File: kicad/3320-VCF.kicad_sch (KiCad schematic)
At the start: 65 parts, among them J1 EuroPower_JST_3P, J2 EURO_PWR_16P, U1 TL072, U2 TL074, U3 AS3320

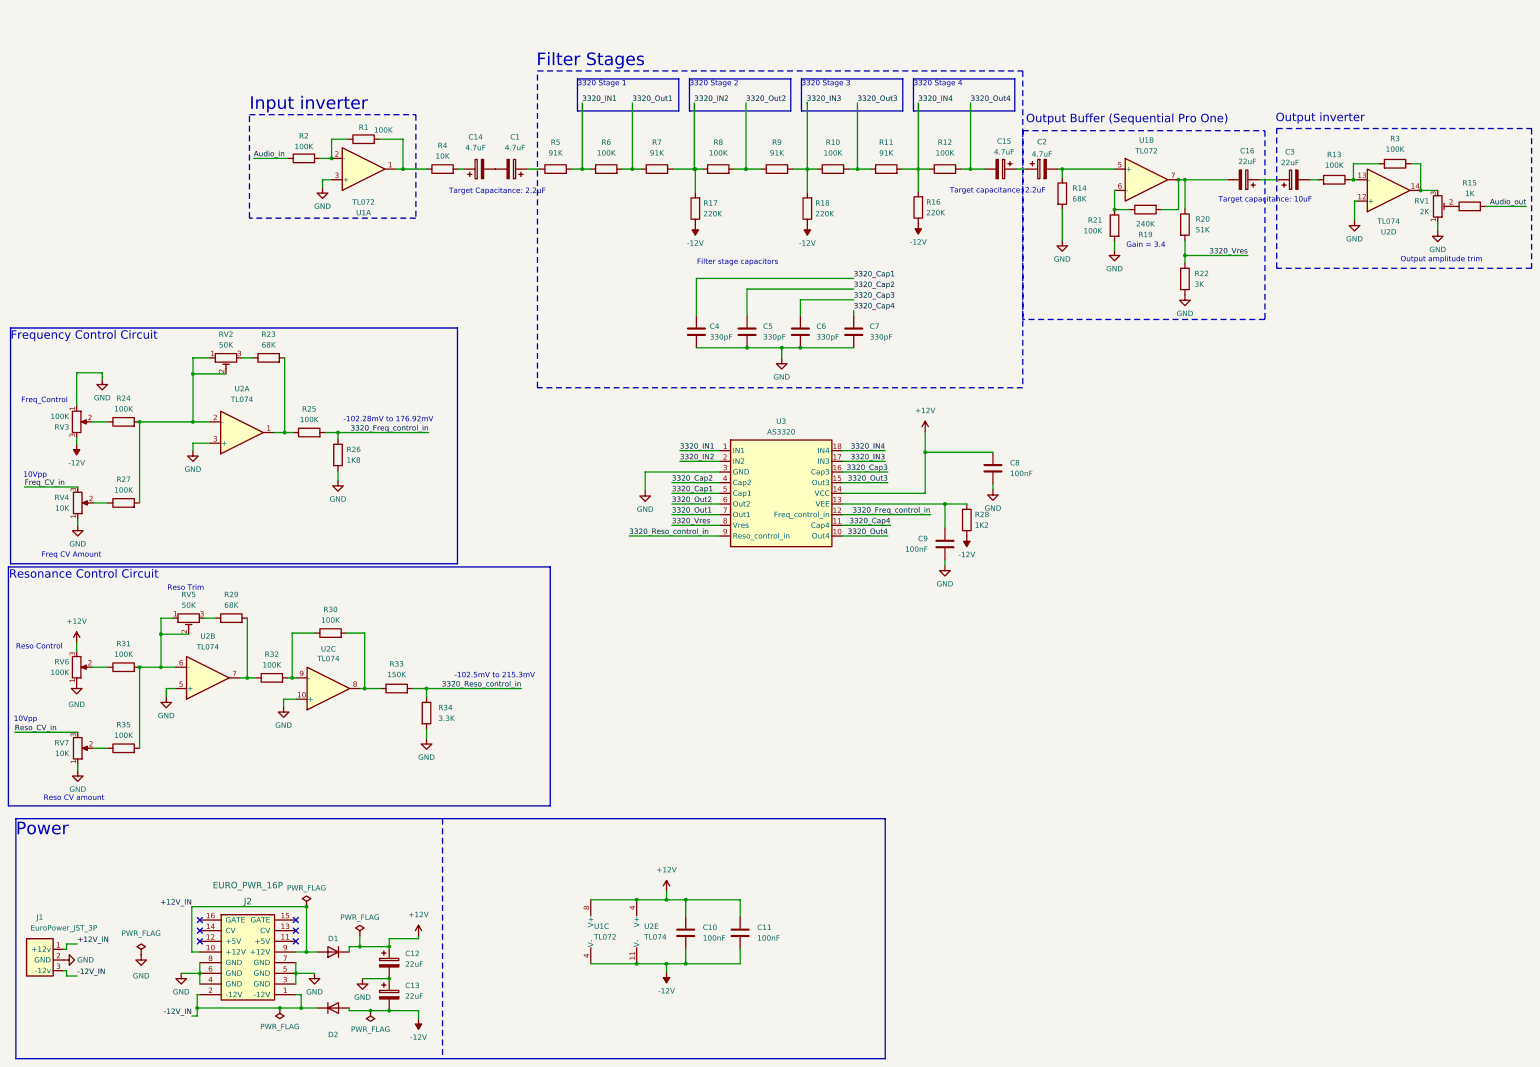
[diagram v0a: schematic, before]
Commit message: Added Schematic Revision 0.1.1
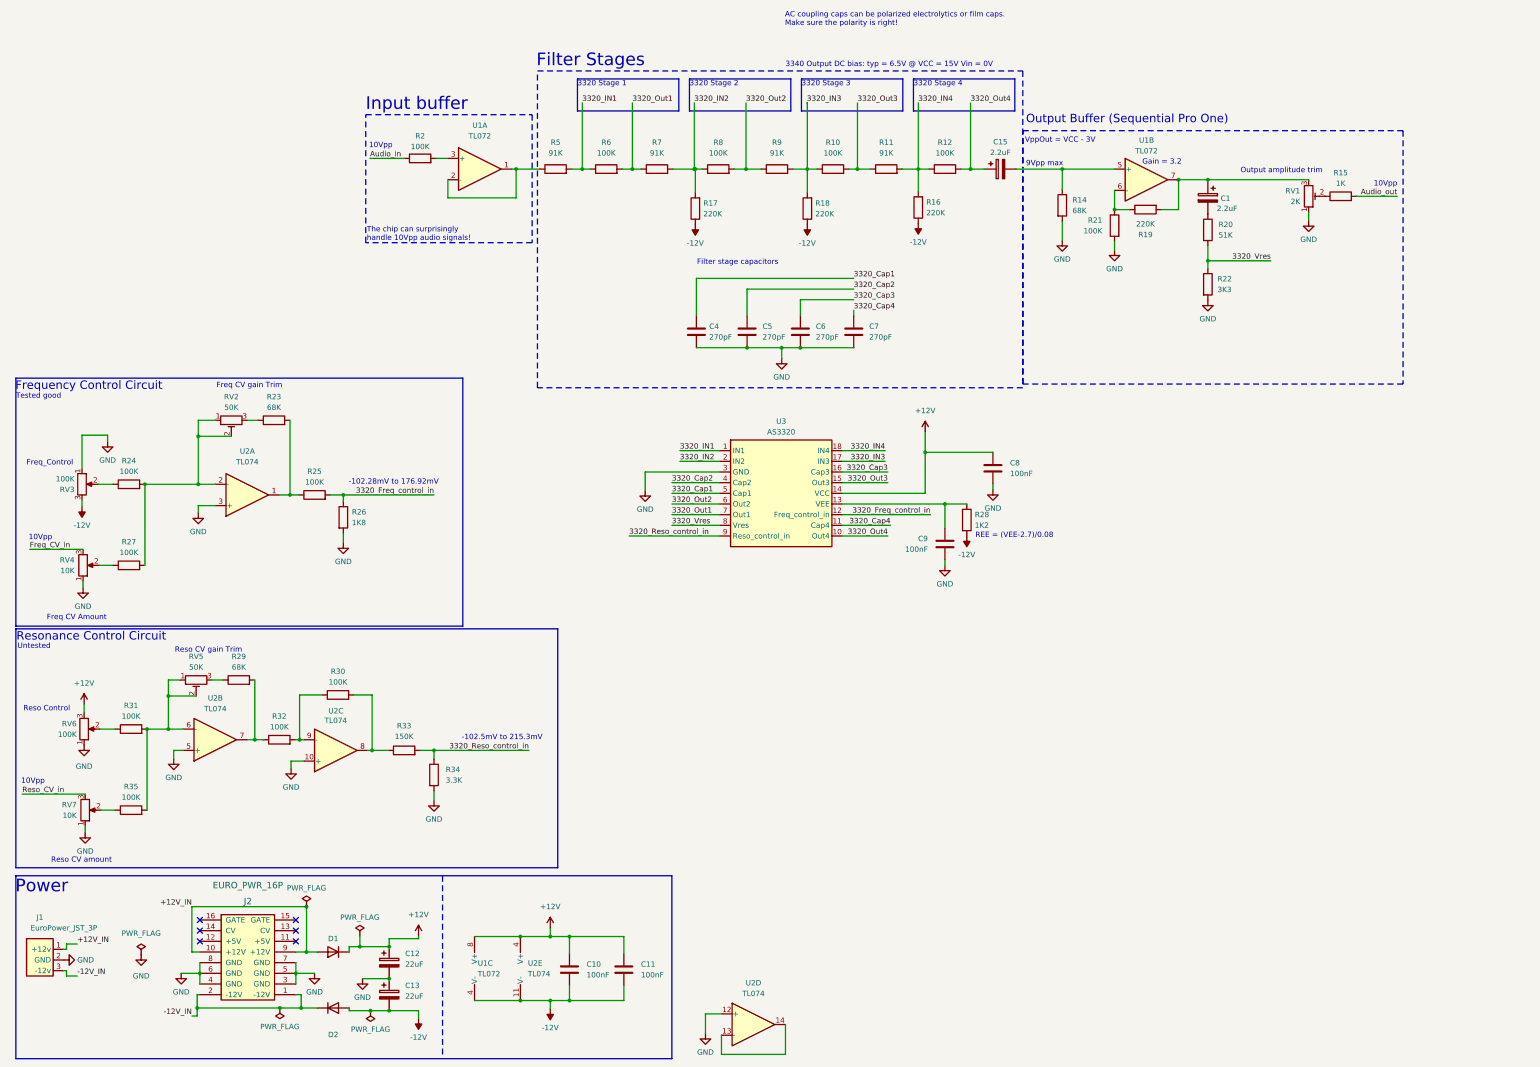
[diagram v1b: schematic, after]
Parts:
- removed C14, C2: 4.7uF, symbol Device:C_Polarized
- removed C16, C3: 22uF, symbol Device:C_Polarized
- removed R1, R13, R3: 100K, symbol Device:R
- removed R4: 10K, symbol Device:R
- C1, C15: value 4.7uF -> 2.2uF
- C4, C5, C6, C7: value 330pF -> 270pF
- R19: value 240K -> 220K
- R22: value 3K -> 3K3
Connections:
- net 3320_Out4: now also C15.1; no longer C15.2
- net GND: no longer U1.3 (+)
- net at R14.1, U1.5 (+): now also C15.2
- net at C1.2: now also R20.1
- net at U1.1: now also R5.1, U1.2 (-)
- net at U2.13 (-): now also U2.14
- net at C1.1: now also R19.2, RV1.3, U1.7; no longer R5.1
- net at R2.2: now also U1.3 (+); no longer U1.2 (-)
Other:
- note added: "3340 Output DC bias: typ = 6.5V @ VCC = 15V Vin = 0V"
- note added: "9Vpp max"
- note added: "AC coupling caps can be polarized electrolytics or film caps. Make sure the polarity is right!"
- note added: "Freq CV gain Trim"
- note added: "Gain = 3.2"
- note added: "Input buffer"
- note added: "REE = (VEE-2.7)/0.08"
- note added: "Reso CV gain Trim"
- note added: "Tested good"
- note added: "The chip can surprisingly handle 10Vpp audio signals!"
- note added: "Untested"
- note added: "VppOut = VCC - 3V"
- note removed: "Gain = 3.4"
- note removed: "Input inverter"
- note removed: "Output inverter"
- note removed: "Reso Trim"
- note removed: "Target Capacitance: 2.2uF"
- note removed: "Target capacitance: 10uF"
- note removed: "Target capacitance: 2.2uF"
- moved on the sheet: C10, C11, C15, R14, R15, R2, R20, R22, R23, R24, R25, R26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
